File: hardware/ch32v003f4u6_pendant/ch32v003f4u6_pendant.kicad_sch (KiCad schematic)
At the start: 52 parts, among them J1 USB_C_Receptacle_USB2.0, J2 BONUS, J3 BONUS, J4 CONN, J7 BATT, Q1 Q_Photo_NPN, Q2 NMOS, T1 TOUCHPAD, U1 MD5112, U2 CH32V003F4U6, U3 MD5112, U4 QMA7981, U5 RY2200, U6 RS3236-3.3YUTDN4, U7 S08OB383-031

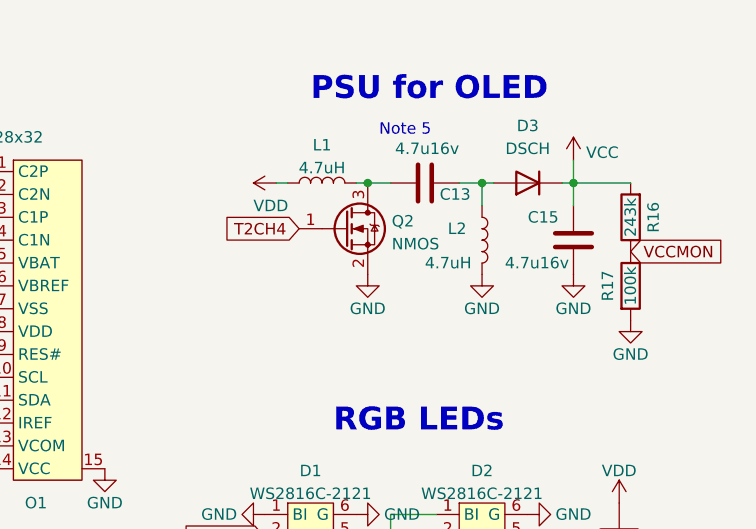
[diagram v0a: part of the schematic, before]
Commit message: Update design a little
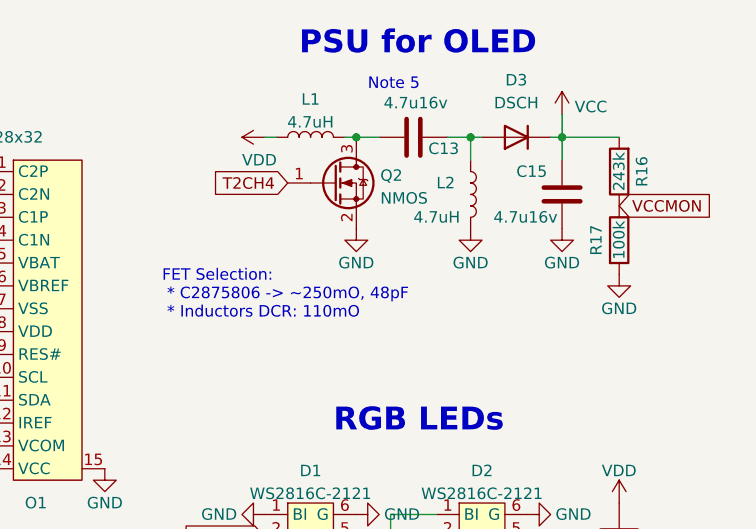
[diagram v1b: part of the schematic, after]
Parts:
- Q2: footprint Package_TO_SOT_SMD:SOT-323_SC-70 -> DFN-3L-1x0.6:DFN-3L-1x0.6; LCSC C719079 -> C2875806
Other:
- note added: "FET Selection: * C2875806 -> ~250mO, 48pF * Inductors DCR: 110mO"
- moved on the sheet: C13, C15, D3, L1, L2, Q2, R16, R17
